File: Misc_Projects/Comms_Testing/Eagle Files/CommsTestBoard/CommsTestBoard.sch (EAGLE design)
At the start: 12 parts, among them J1 1985205, J2 1985205

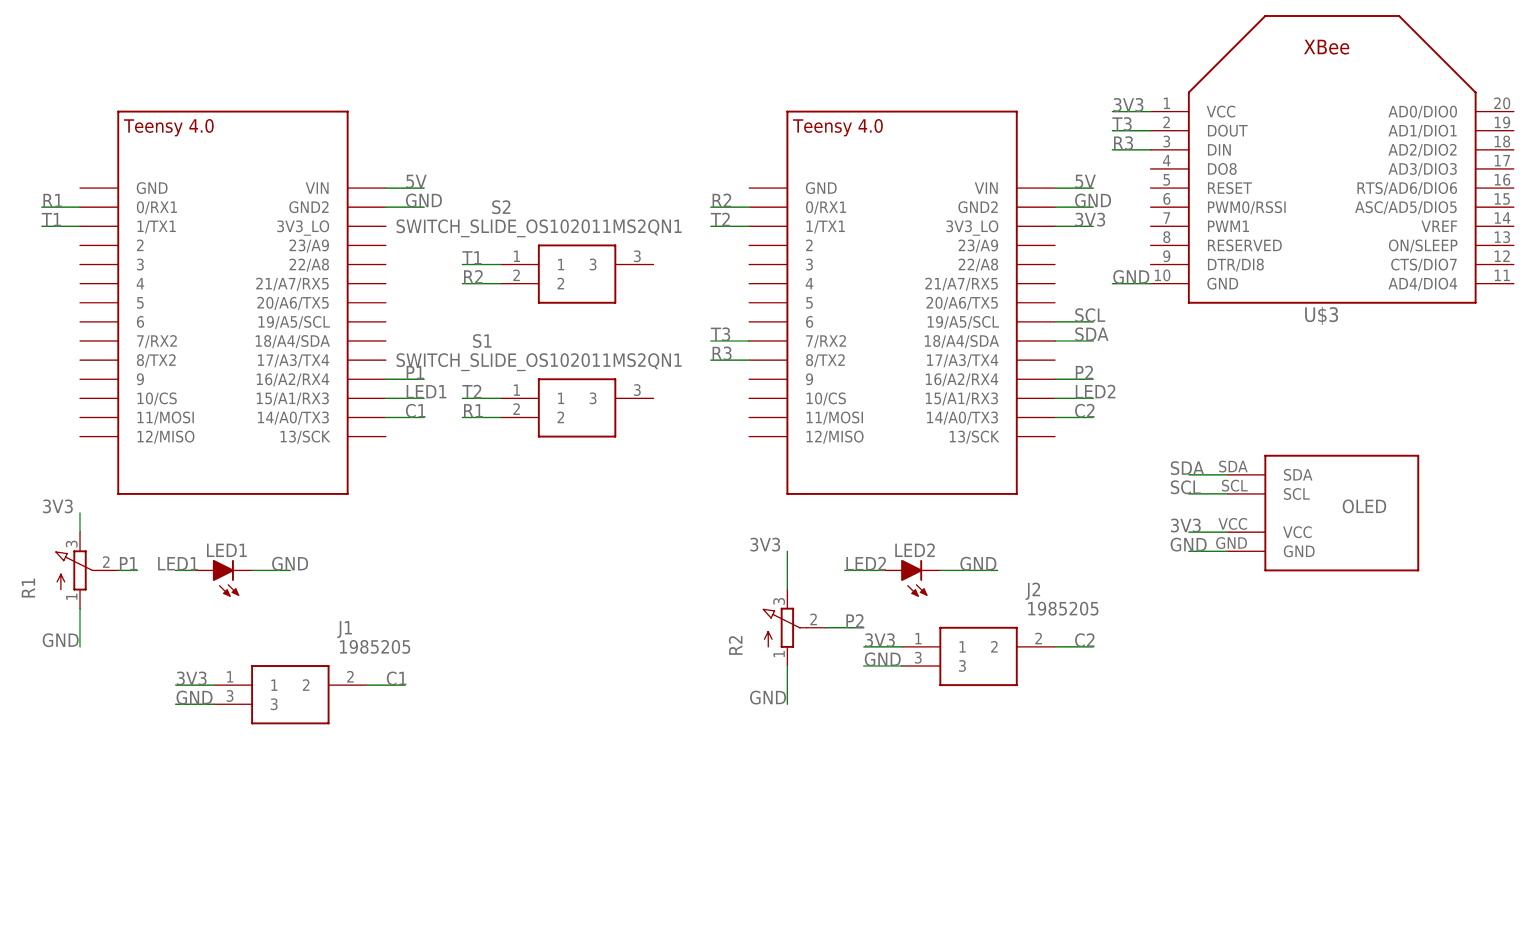
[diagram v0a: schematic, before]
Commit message: Updated comms testing board
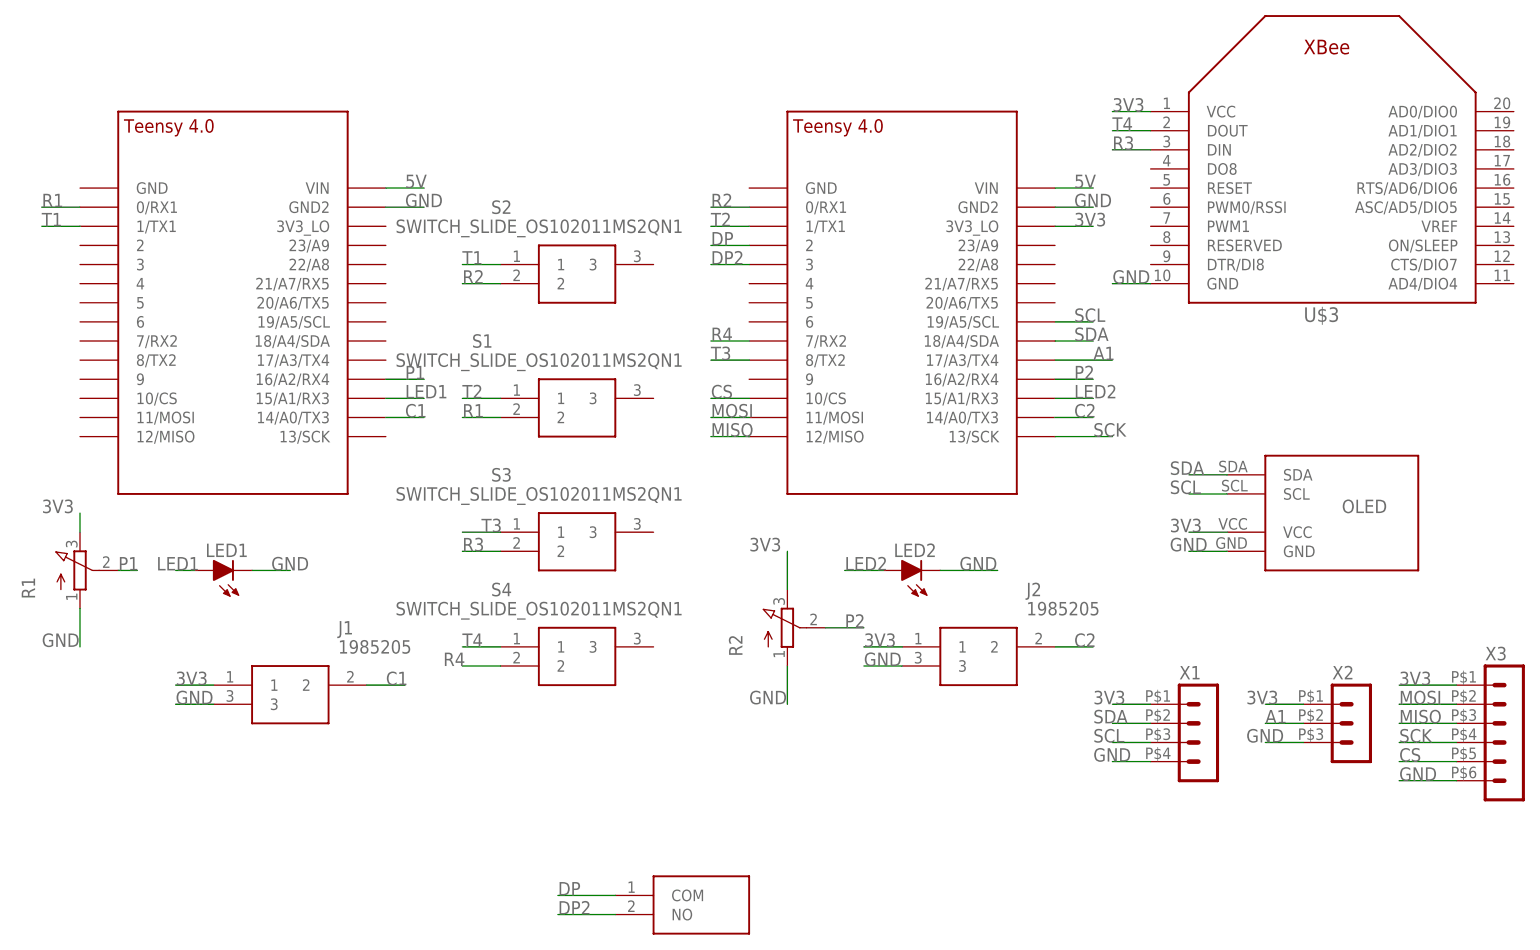
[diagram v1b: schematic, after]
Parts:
- added S3, S4: SWITCH_SLIDE_OS102011MS2QN1, GTOR - Active Components:SWITCH_SLIDE_OS102011MS2QN1
- added S5: PTS636_SL50_LFS, GTOR - Active Components:PTS636_SL50_LFS
- added X1: (no value), GTOR - Microfit Connector:HEADER_POS4_43045-0401
- added X2: (no value), GTOR - Microfit Connector:HEADER_POS3_43650-0300
- added X3: (no value), GTOR - Microfit Connector:HEADER_POS6_43045-0600
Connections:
- new net A1: U$2.17/A3/TX4, X2.2
- new net CS: U$2.10/CS, X3.5
- new net DP: S5.COM, U$2.2
- new net DP2: S5.NO, U$2.3
- new net MISO: U$2.12/MISO, X3.3
- new net MOSI: U$2.11/MOSI, X3.2
- new net R4: S4.2, U$2.7/RX2
- new net SCK: U$2.13/SCK, X3.4
- new net T4: S4.1, U$3.DOUT
- net 3V3: now also X1.1, X2.1, X3.1
- net GND: now also X1.4, X2.3, X3.6
- net R3: now also S3.2; no longer U$2.8/TX2
- net SCL: now also X1.3
- net SDA: now also X1.2
- net T3: now also S3.1, U$2.8/TX2; no longer U$2.7/RX2, U$3.DOUT
